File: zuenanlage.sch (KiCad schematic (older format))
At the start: 0 parts

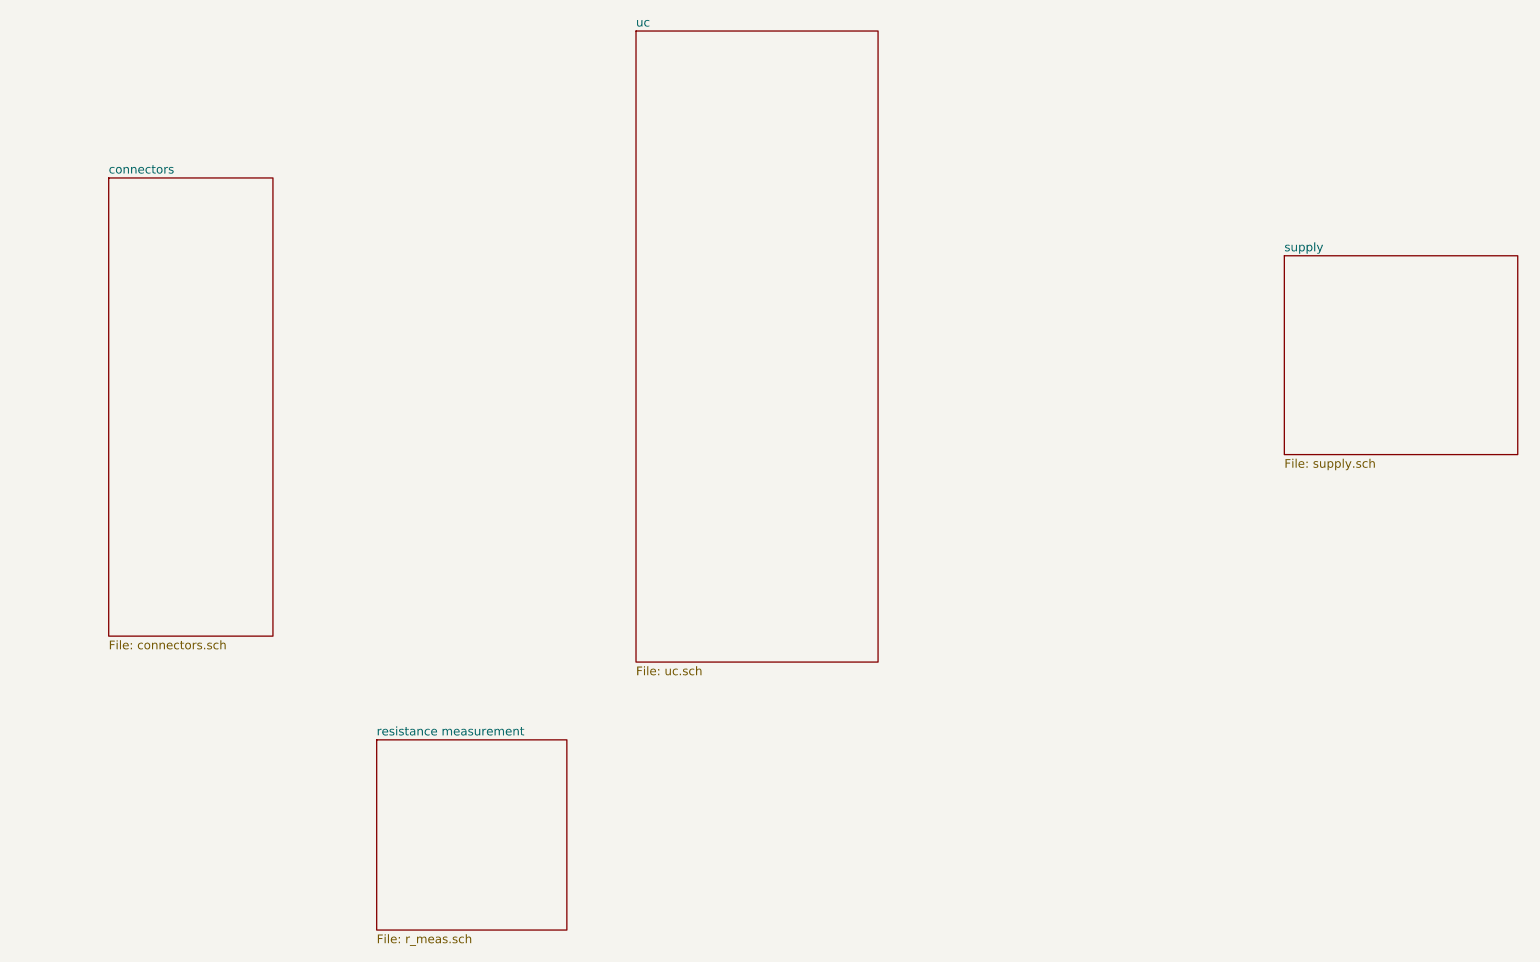
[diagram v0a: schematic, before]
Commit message: finished schematic for review
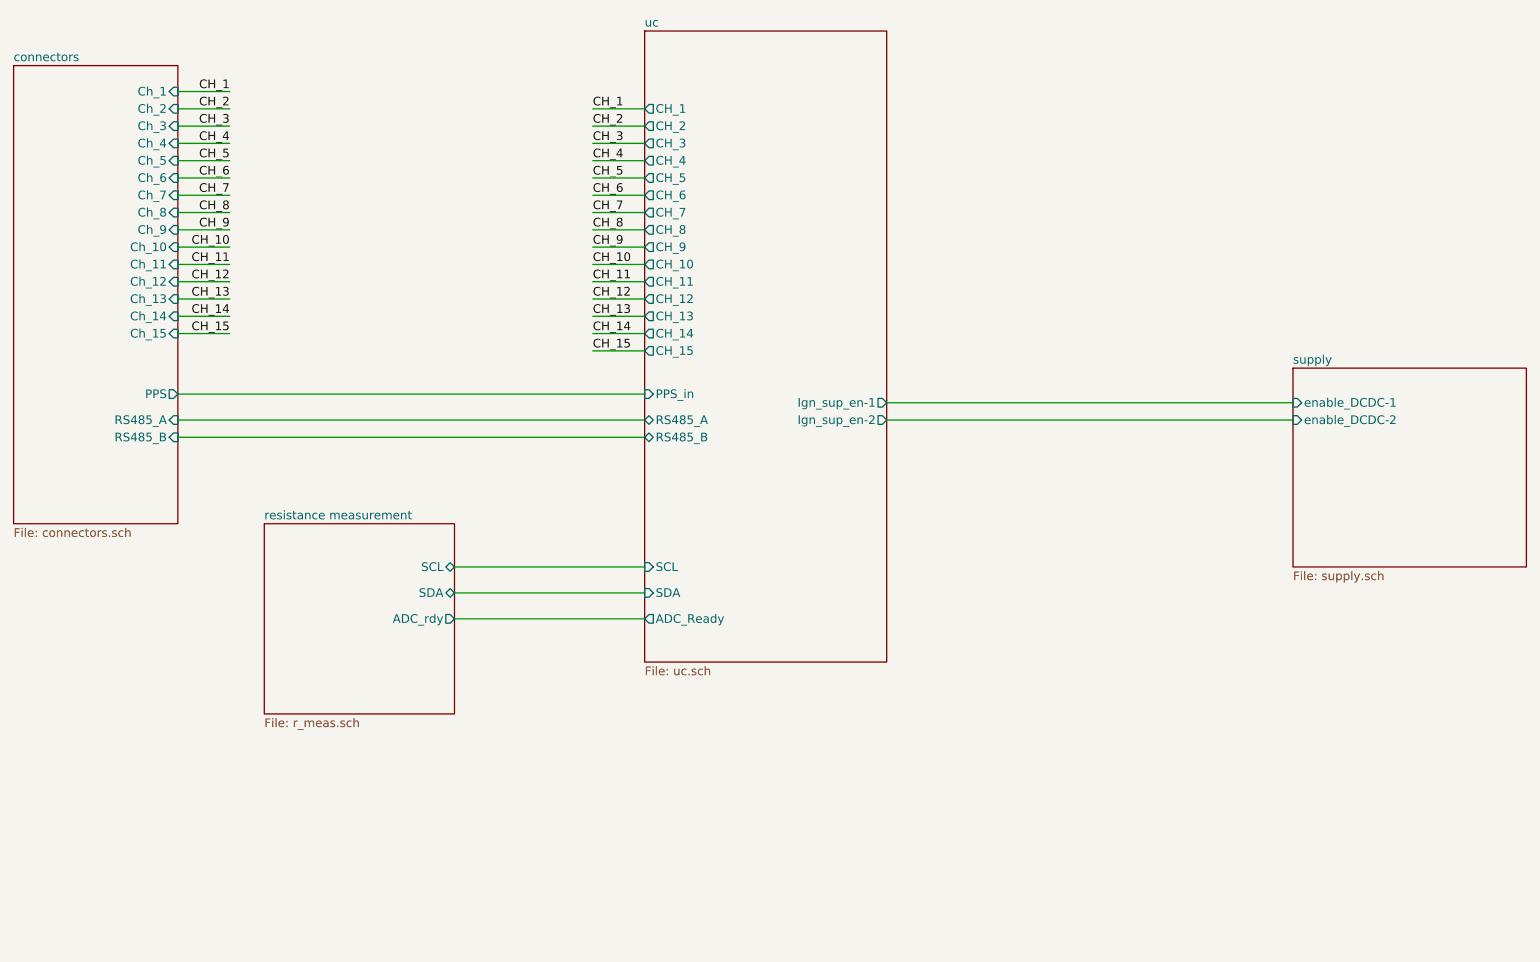
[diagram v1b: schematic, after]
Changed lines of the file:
@@
 $EndDescr
 $Sheet
-S 4850 1600 1400 3650
+S 4900 1600 1400 3650
 U 5D1E53B8
 F0 "uc" 50
 F1 "uc.sch" 50
-$EndSheet
-$Sheet
-S 8600 2900 1350 1150
+F2 "CH_1" O L 4900 2050 50
+F3 "CH_2" O L 4900 2150 50
+F4 "CH_3" O L 4900 2250 50
+F5 "CH_4" O L 4900 2350 50
+F6 "CH_5" O L 4900 2450 50
+F7 "CH_6" O L 4900 2550 50
+F8 "CH_7" O L 4900 2650 50
+F9 "CH_8" O L 4900 2750 50
+F10 "CH_9" O L 4900 2850 50
+F11 "CH_10" O L 4900 2950 50
+F12 "CH_11" O L 4900 3050 50
+F13 "CH_12" O L 4900 3150 50
+F14 "CH_13" O L 4900 3250 50
+F15 "CH_14" O L 4900 3350 50
+F16 "CH_15" O L 4900 3450 50
+F17 "Ign_sup_en-1" O R 6300 3750 50
+F18 "Ign_sup_en-2" O R 6300 3850 50
+F19 "PPS_in" I L 4900 3700 50
+F20 "RS485_B" B L 4900 3950 50
+F21 "RS485_A" B L 4900 3850 50
+F22 "SDA" I L 4900 4850 50
+F23 "SCL" I L 4900 4700 50
+F24 "ADC_Ready" O L 4900 5000 50
+$EndSheet
+$Sheet
+S 8650 3550 1350 1150
 U 5D2135F9
 F0 "supply" 50
 F1 "supply.sch" 50
-$EndSheet
-$Sheet
-S 1800 2450 950  2650
+F2 "enable_DCDC-1" I L 8650 3750 50
+F3 "enable_DCDC-2" I L 8650 3850 50
+$EndSheet
+$Sheet
+S 1250 1800 950  2650
 U 5D36F340
 F0 "connectors" 50
 F1 "connectors.sch" 50
-$EndSheet
-$Sheet
-S 3350 5700 1100 1100
+F2 "Ch_5" I R 2200 2350 50
+F3 "Ch_6" I R 2200 2450 50
+F4 "Ch_7" I R 2200 2550 50
+F5 "Ch_8" I R 2200 2650 50
+F6 "Ch_1" I R 2200 1950 50
+F7 "Ch_2" I R 2200 2050 50
+F8 "Ch_3" I R 2200 2150 50
+F9 "Ch_4" I R 2200 2250 50
+F10 "Ch_9" I R 2200 2750 50
+F11 "Ch_10" I R 2200 2850 50
+F12 "Ch_11" I R 2200 2950 50
+F13 "Ch_12" I R 2200 3050 50
+F14 "PPS" O R 2200 3700 50
+F15 "Ch_13" I R 2200 3150 50
+F16 "Ch_14" I R 2200 3250 50
+F17 "Ch_15" I R 2200 3350 50
+F18 "RS485_A" I R 2200 3850 50
+F19 "RS485_B" I R 2200 3950 50
+$EndSheet
+$Sheet
+S 2700 4450 1100 1100
 U 5D5C8F4D
 F0 "resistance measurement" 50
 F1 "r_meas.sch" 50
-$EndSheet
+F2 "SCL" B R 3800 4700 50
+F3 "SDA" B R 3800 4850 50
+F4 "ADC_rdy" O R 3800 5000 50
+$EndSheet
+Wire Wire Line
+	2200 3700 4900 3700
+Wire Wire Line
+	2200 3850 4900 3850
+Wire Wire Line
+	2200 3950 4900 3950
+Wire Wire Line
+	2200 3350 2500 3350
+Text Label 2500 3350 2    50   ~ 0
+CH_15
+Wire Wire Line
+	2200 3250 2500 3250
+Text Label 2500 3250 2    50   ~ 0
+CH_14
+Wire Wire Line
+	2200 3150 2500 3150
+Text Label 2500 3150 2    50   ~ 0
+CH_13
+Wire Wire Line
+	2200 3050 2500 3050
+Text Label 2500 3050 2    50   ~ 0
+CH_12
+Wire Wire Line
+	2200 2950 2500 2950
+Text Label 2500 2950 2    50   ~ 0
+CH_11
+Wire Wire Line
+	2200 2850 2500 2850
+Text Label 2500 2850 2    50   ~ 0
+CH_10
+Wire Wire Line
+	2200 2750 2500 2750
+Text Label 2500 2750 2    50   ~ 0
+CH_9
+Wire Wire Line
+	2200 2650 2500 2650
+Text Label 2500 2650 2    50   ~ 0
+CH_8
+Wire Wire Line
+	2200 2550 2500 2550
+Text Label 2500 2550 2    50   ~ 0
+CH_7
+Wire Wire Line
+	2200 2450 2500 2450
+Text Label 2500 2450 2    50   ~ 0
+CH_6
+Wire Wire Line
+	2200 2350 2500 2350
+Text Label 2500 2350 2    50   ~ 0
+CH_5
+Wire Wire Line
+	2200 2250 2500 2250
+Text Label 2500 2250 2    50   ~ 0
+CH_4
+Wire Wire Line
+	2200 2150 2500 2150
+Text Label 2500 2150 2    50   ~ 0
+CH_3
+Wire Wire Line
+	2200 2050 2500 2050
+Text Label 2500 2050 2    50   ~ 0
+CH_2
+Wire Wire Line
+	2200 1950 2500 1950
+Text Label 2500 1950 2    50   ~ 0
+CH_1
+Wire Wire Line
+	4900 3450 4600 3450
+Text Label 4600 3450 0    50   ~ 0
+CH_15
+Wire Wire Line
+	4900 3350 4600 3350
+Text Label 4600 3350 0    50   ~ 0
+CH_14
+Wire Wire Line
+	4900 3250 4600 3250
+Text Label 4600 3250 0    50   ~ 0
+CH_13
+Wire Wire Line
+	4900 3150 4600 3150
+Text Label 4600 3150 0    50   ~ 0
+CH_12
+Wire Wire Line
+	4900 3050 4600 3050
+Text Label 4600 3050 0    50   ~ 0
+CH_11
+Wire Wire Line
+	4900 2950 4600 2950
+Text Label 4600 2950 0    50   ~ 0
+CH_10
+Wire Wire Line
+	4900 2850 4600 2850
+Text Label 4600 2850 0    50   ~ 0
+CH_9
+Wire Wire Line
+	4900 2750 4600 2750
+Text Label 4600 2750 0    50   ~ 0
+CH_8
+Wire Wire Line
+	4900 2650 4600 2650
+Text Label 4600 2650 0    50   ~ 0
+CH_7
+Wire Wire Line
+	4900 2550 4600 2550
+Text Label 4600 2550 0    50   ~ 0
+CH_6
+Wire Wire Line
+	4900 2450 4600 2450
+Text Label 4600 2450 0    50   ~ 0
+CH_5
+Wire Wire Line
+	4900 2350 4600 2350
+Text Label 4600 2350 0    50   ~ 0
+CH_4
+Wire Wire Line
+	4900 2250 4600 2250
+Text Label 4600 2250 0    50   ~ 0
+CH_3
+Wire Wire Line
+	4900 2150 4600 2150
+Text Label 4600 2150 0    50   ~ 0
+CH_2
+Wire Wire Line
+	4900 2050 4600 2050
+Text Label 4600 2050 0    50   ~ 0
+CH_1
+Wire Wire Line
+	6300 3750 8650 3750
+Wire Wire Line
+	6300 3850 8650 3850
+Wire Wire Line
+	3800 4700 4900 4700
+Wire Wire Line
+	3800 4850 4900 4850
+Wire Wire Line
+	3800 5000 4900 5000
 $EndSCHEMATC
